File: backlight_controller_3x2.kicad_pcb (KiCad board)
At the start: 2 copper layers, 70.5 x 41.9 mm, 38 parts, among them J1 DB9F_SMD, J2 DB9M_SMD, J3 M12-5_RCPT_F, J4 M12-5_RCPT_F, P1 MINI_FIT_JR_02X03_M_RA, U1 SN74ABT541BDWR, U2 SN74ABT541BDWR

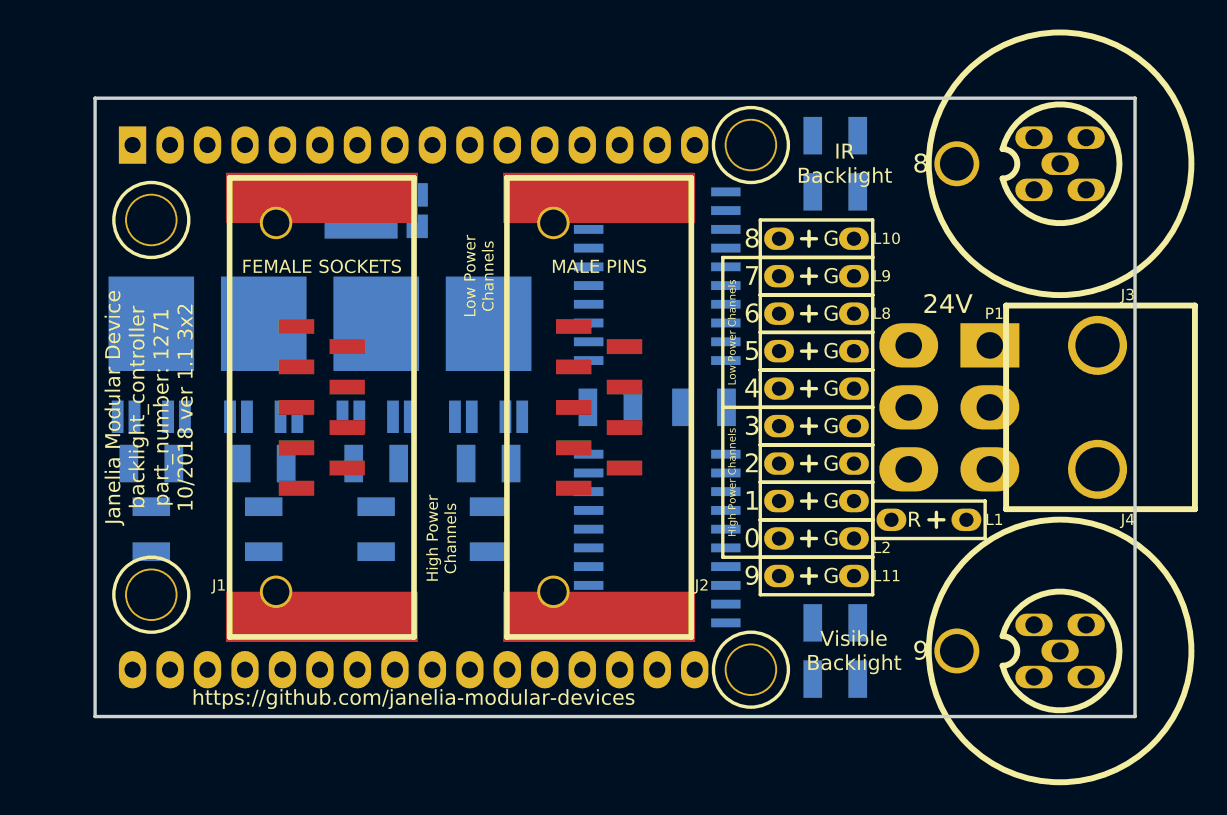
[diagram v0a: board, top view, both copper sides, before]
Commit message: Finished version 1.1.
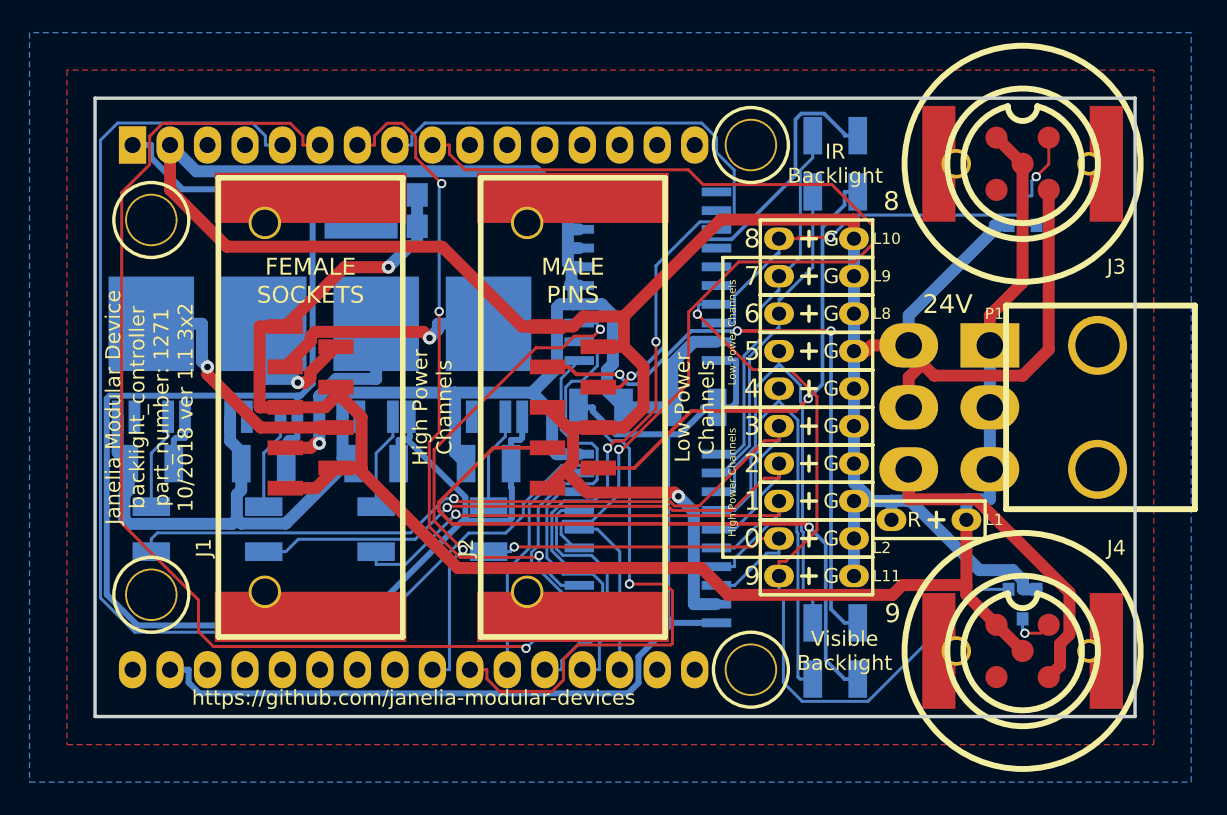
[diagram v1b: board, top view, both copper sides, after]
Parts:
- added U3: NUD3124, backlight_controller_3x2:TO-236-3, B.Cu at (148.6, 75.6)
- added U4: NUD3124, backlight_controller_3x2:TO-236-3, B.Cu at (148.6, 102.2)
- J3, J4: value M12-5_RCPT_F -> M12-5-RCPT_F_SMD; footprint backlight_controller_3x2:M12-5_RCPT_F -> footprints:M12-5_RCPT_F_SMD
- moved J3 2.54 mm to (148.6, 72.4), turned to 0 degrees
- moved J4 2.54 mm to (148.6, 105.4), turned to 0 degrees
- moved J2 1.78 mm to (118.1, 88.9)
- moved J1 0.76 mm to (100.3, 88.9)
- moved C1 0.64 mm to (120.0, 88.9)
- moved C2 0.64 mm to (126.4, 88.9)
- moved U1 0.64 mm to (123.2, 97.8)
- moved U2 0.64 mm to (123.2, 80.0)
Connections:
- J3 pad 2: (no net) -> /backlight_3x2/backlight_outputs/ir/NPN
- J3 pad 4: /backlight_3x2/C_8 -> (no net)
- J4 pad 2: (no net) -> /backlight_3x2/backlight_outputs/visible/NPN
- J4 pad 4: /backlight_3x2/C_9 -> (no net)
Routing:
- net GND: track 0.00 -> 331.0 mm, vias 0 -> 1
- net VAA: track 0.00 -> 124.0 mm, vias 0 -> 1
- net VDD: track 0.00 -> 117.6 mm
- net /~ENABLE: track 0.00 -> 109.7 mm
- net /CHANNEL_0: track 0.00 -> 80.4 mm, vias 0 -> 1
- net VEE: track 0.00 -> 71.0 mm
- net /CHANNEL_3: track 0.00 -> 69.6 mm, vias 0 -> 1
- net /CHANNEL_2: track 0.00 -> 61.8 mm, vias 0 -> 2
- net /backlight_3x2/C_3: track 0.00 -> 57.1 mm, vias 0 -> 1
- net /backlight_3x2/C_9: track 0.00 -> 52.1 mm, vias 0 -> 1
- net /backlight_3x2/low_power_outputs/OUTPUT_0: track 0.00 -> 47.2 mm, vias 0 -> 1
- net /backlight_3x2/C_2: track 0.00 -> 46.4 mm, vias 0 -> 1
- net /CHANNEL_8: track 0.00 -> 46.0 mm, vias 0 -> 1
- net /CHANNEL_1: track 0.00 -> 45.0 mm, vias 0 -> 3
- net /backlight_3x2/low_power_outputs/OUTPUT_1: track 0.00 -> 42.3 mm, vias 0 -> 3
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- added copper zone on B.Cu, net GND
- added copper zone on F.Cu, net VAA
